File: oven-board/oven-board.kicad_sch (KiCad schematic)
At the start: 27 parts, among them J1 temp_sensor, J2 heating element, J3 wall outlet, J4 12V Power Supply, K1 G2RL-1A-E, SW1 SW_Push, SW2 SW_Push, SW3 SW_Push, SW4 SW_Push, SW5 SW_Push, U3 NUCLEO-L432KC, U4 SZNUD3124LT1G, U5 NHD-C0220BIZ, U6 INA826AIDR

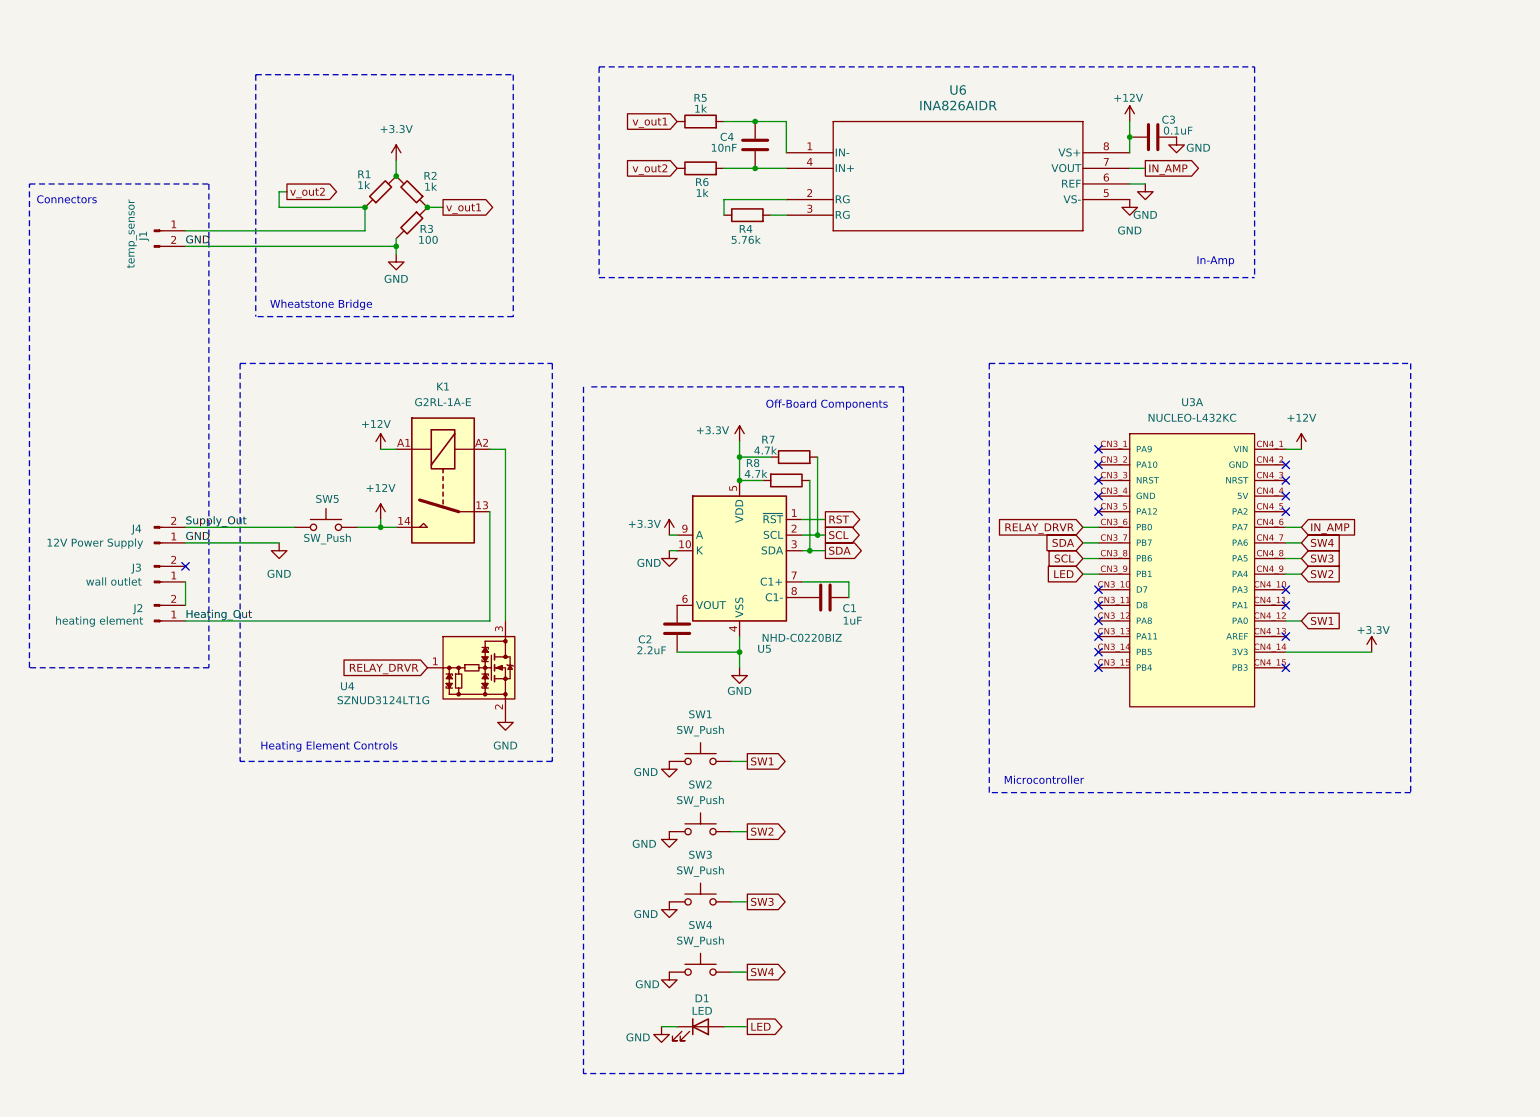
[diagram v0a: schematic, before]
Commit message: Oven Board Rev 2.1
Made all requested changes
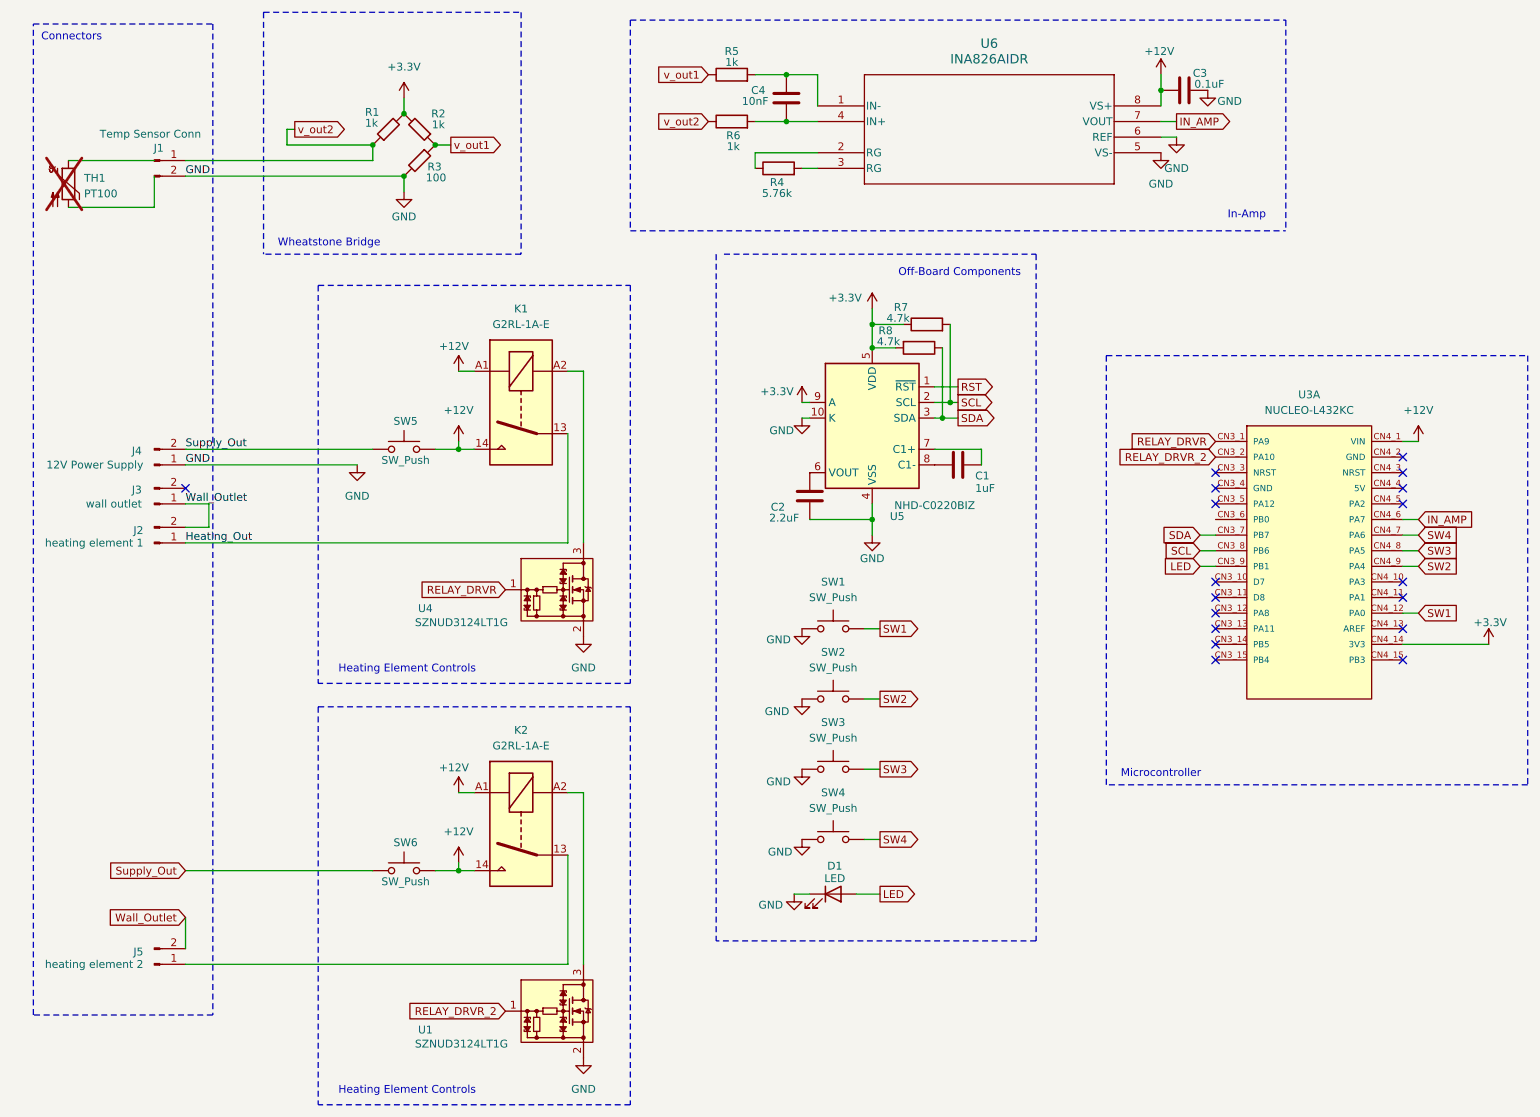
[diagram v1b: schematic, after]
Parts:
- added J5: heating element 2, Library:CONN_1890963_PXC, symbol Connector:Conn_01x02_Pin
- added K2: G2RL-1A-E, Library:RELAY_G2RL-1A-E DC5_OMR, symbol Relay:G2RL-1A-E
- added SW6: SW_Push, Library:SW_PB300STQ, symbol Switch:SW_Push
- added TH1: PT100, symbol Sensor_Temperature:PT100
- added U1: SZNUD3124LT1G, Package_TO_SOT_SMD:TSOT-23_HandSoldering, symbol FS_4_Global_Symbol_Library:SZNUD3124LT1G
- C1: footprint (none) -> Library:CAP_GRM21_MUR_1uF
- C2: footprint (none) -> Library:CAP_CC0805_EB_YAG_2.2uF
- C3: footprint (none) -> Library:CC0805N_YAG_0.1uF
- C4: footprint (none) -> Library:CAPC17595_87N_KEM_10nF
- D1: footprint (none) -> Library:LED_LTL-307E_LTO; Digi PN (none) -> 160-1705-ND; Digi URL (none) -> https://www.digikey.com/en/products/detail/liteon/LTL-307E/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; MFG (none) -> Lite-On Inc.; MFG PN (none) -> LTL-307E
- J1: value temp_sensor -> Temp Sensor Conn; footprint (none) -> Library:CONN_1890963_PXC
- J2: value heating element -> heating element 1; footprint (none) -> Library:CONN_1890963_PXC
- J3, J4: footprint (none) -> Library:CONN_1890963_PXC
- K1: footprint Relay_THT:Relay_SPST_Omron_G2RL-1A-E -> Library:RELAY_G2RL-1A-E DC5_OMR
- R1, R2, R5, R6: footprint (none) -> Library:RC0805N_YAG_1K
- R3: footprint (none) -> Library:RC0805N_YAG_100
- R4: footprint (none) -> Library:RC0603N_YAG_5.76K
- R7, R8: footprint (none) -> Library:RES_RC0805_YAG_4.7K
- SW1, SW2, SW3, SW4, SW5: footprint (none) -> Library:SW_PB300STQ
- U3: Digi PN (none) -> 497-16592-ND; Digi URL (none) -> https://www.digikey.com/en/products/detail/stmicroelectroni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; MFG (none) -> STMicroelectronics; MFG PN (none) -> NUCLEO-L432KC
- U5: footprint Display:NHD-C0220BiZ -> Library:NHD-C0220BIZ-FSW-FBW-3V3M_NDI
- U6: footprint D8 -> Library:INA826AIDR
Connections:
- net +12V: now also K2.14, K2.A1, SW6.1
- net GND: now also U1.2
- net RELAY_DRVR: now also U3.CN3_1 (PA9); no longer U3.CN3_6 (PB0)
- net Supply_Out: now also SW6.2
- net RELAY_DRVR_2: now reaches U3.CN3_2 (PA10)
- net RELAY_DRVR_2: now also U1.1
- net Wall_Outlet: now reaches J2.2 (Pin_2), J3.1 (Pin_1)
- net Wall_Outlet: now also J5.2 (Pin_2)
- new net: J5.1 (Pin_1), K2.13
- new net: K2.A2, U1.3
- no-connect marks 20 -> 18
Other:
- moved on the sheet: C1, C2, C3, C4, D1, J1, J2, J3, J4, K1, R1, R2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
